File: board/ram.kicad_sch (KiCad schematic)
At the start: 16 parts, among them U10 RAM 1 LO, U11 RAM 1 HI, U4 RAM 1 LO, U5 RAM 1 HI, U6 RAM 1 LO, U7 RAM 1 HI, U8 RAM 1 LO, U9 RAM 1 HI

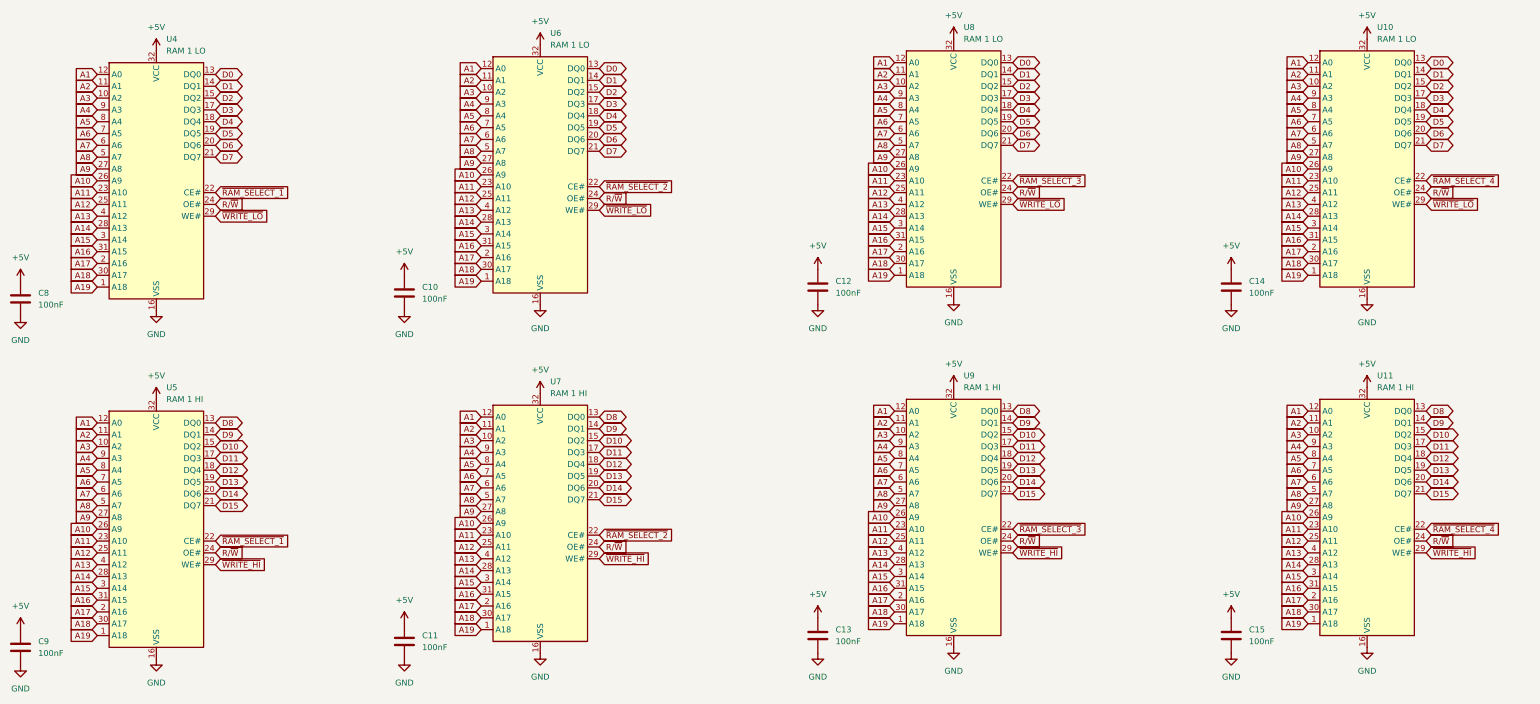
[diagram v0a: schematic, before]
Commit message: design draft complete, added footprints
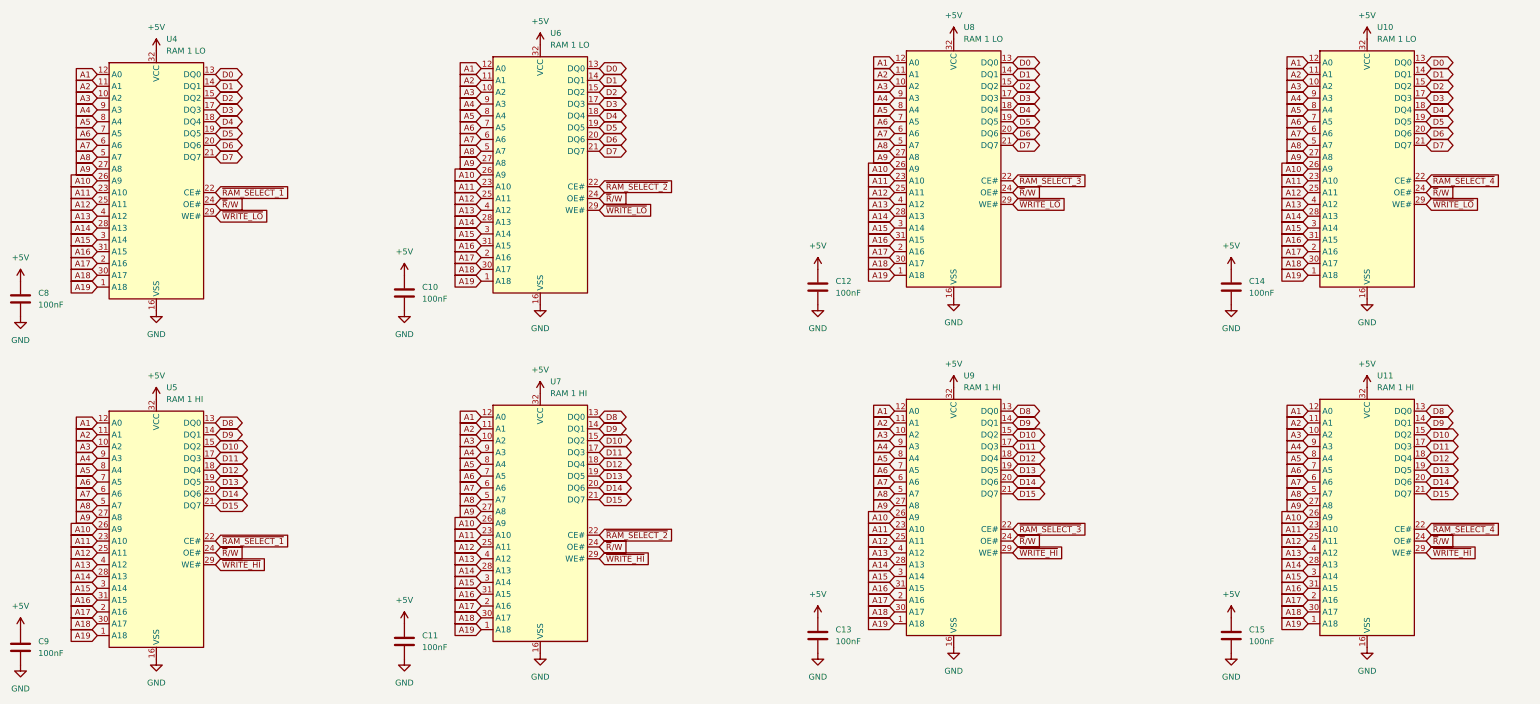
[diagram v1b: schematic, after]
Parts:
- C10, C11, C12, C13, C14, C15, C8, C9: footprint (none) -> Capacitor_THT:C_Disc_D5.0mm_W2.5mm_P5.00mm
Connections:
- net R/~{W} renamed ~{R}/W
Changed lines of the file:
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@@
 		)
 	)
-	(global_label "R{slash}~{W}"
+	(global_label "~{R}{slash}W"
 		(shape input)
 		(at 250.19 165.1 0)
@@
 		)
 	)
-	(global_label "R{slash}~{W}"
+	(global_label "~{R}{slash}W"
 		(shape input)
 		(at 161.29 166.37 0)
@@
 		)
 	)
-	(global_label "R{slash}~{W}"
+	(global_label "~{R}{slash}W"
 		(shape input)
 		(at 339.09 90.17 0)
@@
 		)
 	)
-	(global_label "R{slash}~{W}"
+	(global_label "~{R}{slash}W"
 		(shape input)
 		(at 250.19 90.17 0)
@@
 		)
 	)
-	(global_label "R{slash}~{W}"
+	(global_label "~{R}{slash}W"
 		(shape input)
 		(at 161.29 91.44 0)
@@
 		)
 	)
-	(global_label "R{slash}~{W}"
+	(global_label "~{R}{slash}W"
 		(shape input)
 		(at 339.09 165.1 0)
@@
 		)
 	)
-	(global_label "R{slash}~{W}"
+	(global_label "~{R}{slash}W"
 		(shape input)
 		(at 78.74 92.71 0)
@@
 		)
 	)
-	(global_label "R{slash}~{W}"
+	(global_label "~{R}{slash}W"
 		(shape input)
 		(at 78.74 167.64 0)
@@
 			)
 		)
-		(property "Footprint" ""
+		(property "Footprint" "Capacitor_THT:C_Disc_D5.0mm_W2.5mm_P5.00mm"
 			(at 120.3452 190.5 0)
 			(effects
@@
 			)
 		)
-		(property "Footprint" ""
+		(property "Footprint" "Capacitor_THT:C_Disc_D5.0mm_W2.5mm_P5.00mm"
 			(at 298.1452 189.23 0)
 			(effects
@@
 			)
 		)
-		(property "Footprint" ""
+		(property "Footprint" "Capacitor_THT:C_Disc_D5.0mm_W2.5mm_P5.00mm"
 			(at 120.3452 115.57 0)
 			(effects
@@
 			)
 		)
-		(property "Footprint" ""
+		(property "Footprint" "Capacitor_THT:C_Disc_D5.0mm_W2.5mm_P5.00mm"
 			(at 37.7952 116.84 0)
 			(effects
@@
 			)
 		)
-		(property "Footprint" ""
+		(property "Footprint" "Capacitor_THT:C_Disc_D5.0mm_W2.5mm_P5.00mm"
 			(at 37.7952 191.77 0)
 			(effects
@@
 			)
 		)
-		(property "Footprint" ""
+		(property "Footprint" "Capacitor_THT:C_Disc_D5.0mm_W2.5mm_P5.00mm"
 			(at 298.1452 114.3 0)
 			(effects
@@
 			)
 		)
-		(property "Footprint" ""
+		(property "Footprint" "Capacitor_THT:C_Disc_D5.0mm_W2.5mm_P5.00mm"
 			(at 209.2452 189.23 0)
 			(effects
@@
 			)
 		)
-		(property "Footprint" ""
+		(property "Footprint" "Capacitor_THT:C_Disc_D5.0mm_W2.5mm_P5.00mm"
 			(at 209.2452 114.3 0)
 			(effects
